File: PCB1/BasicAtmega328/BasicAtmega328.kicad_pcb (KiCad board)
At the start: 2 copper layers, 0 parts

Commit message: Placa enrutada
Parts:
- added C1: 47uF, Capacitors_SMD:CP_Elec_6.3x5.7, F.Cu at (110.5, 97.8)
- added C2: 100nF, Capacitors_SMD:C_0805, F.Cu at (104.1, 78.7)
- added C3: 4.7uF, Capacitors_SMD:C_0805, F.Cu at (102.5, 77.1)
- added C5: 100nF, Capacitors_SMD:C_0805, F.Cu at (113.6, 89.5)
- added C6: 100nF, Capacitors_SMD:C_0805, F.Cu at (97.3, 97.6)
- added C7: 10uF, Capacitors_SMD:C_0805, F.Cu at (118.8, 82.0)
- added C8: 100nF, Capacitors_SMD:C_0805, F.Cu at (118.8, 80.1)
- added D1: MBRA140, Diodes_SMD:D_SMA_Standard, F.Cu at (121.5, 93.0)
- added D2: POWER_ON, LEDs:LED_0805, B.Cu at (113.0, 105.4)
- added D3: SMBJ6.0CA, Diode_SMD:D_SMB, B.Cu at (117.4, 71.3)
- added D4: SMBJ6.0CA, Diode_SMD:D_SMB, B.Cu at (109.1, 71.3)
- added D5: SMBJ6.0CA, Diode_SMD:D_SMB, B.Cu at (100.8, 71.3)
- added F1: 160mA, Fuses:1206, B.Cu at (123.4, 66.4)
- added F2: 160mA, Fuses:1206, B.Cu at (94.7, 66.3)
- added J1: Jack-DC-IN, Connectors:BARREL_JACK, F.Cu at (118.8, 97.0)
- added JP1: VCC_CUT, Jumpers:SMT-JUMPER_2_NO_NO-SILK, B.Cu at (97.5, 84.7)
- added JP2: VCC_CUT, Jumpers:SMT-JUMPER_2_NO_NO-SILK, B.Cu at (119.1, 80.4)
- added JP3: VCC_CUT, Jumpers:SMT-JUMPER_2_NO_NO-SILK, B.Cu at (100.6, 104.3)
- added P1: ISCP, Connectors:2X3, F.Cu at (94.9, 89.3)
- added P2: HEADER1, Pin_Headers:Pin_Header_Straight_1x15, F.Cu at (88.4, 64.2)
- added P3: MODBUS_1, Connectors_Molex:Molex_Microfit3_Header_02x03_Angled_43045-060x, F.Cu at (113.7, 63.4)
- added P4: SERIAL_DEBUG, Connectors_JST:JST_PH_S4B-PH-K_04x2.00mm_Angled, F.Cu at (102.5, 105.0)
- added P5: MODBUS_2, Connectors_Molex:Molex_Microfit3_Header_02x03_Angled_43045-060x, F.Cu at (97.9, 63.4)
- added P6: HEADER2, Pin_Headers:Pin_Header_Straight_1x15, F.Cu at (129.4, 64.4)
- added R1: 1k, Resistors_SMD:R_0805, B.Cu at (113.0, 103.5)
- added R2: 10k, Resistors_SMD:R_0805, F.Cu at (108.1, 74.0)
- added R3: 10k, Resistors_SMD:R_0805, F.Cu at (108.1, 75.9)
- added R4: 1k, Resistors_SMD:R_0805, F.Cu at (98.6, 104.6)
- added R5: 10k, Resistors_SMD:R_0805, F.Cu at (124.1, 73.9)
- added R6: 10k, Resistors_SMD:R_0805, F.Cu at (122.2, 69.8)
- added R7: 10k, Resistors_SMD:R_0805, F.Cu at (111.7, 75.4)
- added R8: 120R(NC), Resistors_SMD:R_0805, B.Cu at (115.3, 73.8)
- added SW1: RESET_Button, Buttons_Switches_SMD:SW_SPST_B3U-3000P, F.Cu at (95.0, 105.1)
- added U1: LM1117-5.0, TO_SOT_Packages_SMD:SOT-223-3_TabPin2, F.Cu at (102.6, 97.9)
- added U2: ATMEGA328P-AU, Housings_QFP:TQFP-32_7x7mm_Pitch0.8mm, F.Cu at (108.1, 84.8)
- added U3: MAX13487E, Housings_SOIC:SO-8_5.3x6.2mm_Pitch1.27mm, F.Cu at (117.9, 75.7)
- added Y1: 16Mhz, Clocks:RESONATOR-SMD-3.2X1.3, F.Cu at (101.2, 81.5)
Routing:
- net +5V: track 0.00 -> 131.6 mm, vias 0 -> 5
- net +12V: track 0.00 -> 102.0 mm, vias 0 -> 3
- net RST: track 0.00 -> 95.8 mm, vias 0 -> 5
- net TXD: track 0.00 -> 59.0 mm, vias 0 -> 2
- net RXD: track 0.00 -> 58.1 mm, vias 0 -> 3
- net 485_TX: track 0.00 -> 49.6 mm, vias 0 -> 3
- net D13-SCK: track 0.00 -> 49.0 mm, vias 0 -> 7
- net 485_RX: track 0.00 -> 41.1 mm, vias 0 -> 2
- net Net-(D4-Pad2): track 0.00 -> 32.3 mm, vias 0 -> 2
- net D12-MISO: track 0.00 -> 31.0 mm
- net D11-MOSI: track 0.00 -> 29.5 mm, vias 0 -> 1
- net Net-(D3-Pad2): track 0.00 -> 28.6 mm, vias 0 -> 3
- net A6: track 0.00 -> 26.0 mm, vias 0 -> 2
- net A7: track 0.00 -> 25.4 mm, vias 0 -> 2
- net D10: track 0.00 -> 25.0 mm
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- added copper zone on B.Cu, net GND
- added copper zone on F.Cu, net GND
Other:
- board outline added: 45 x 49.9 mm

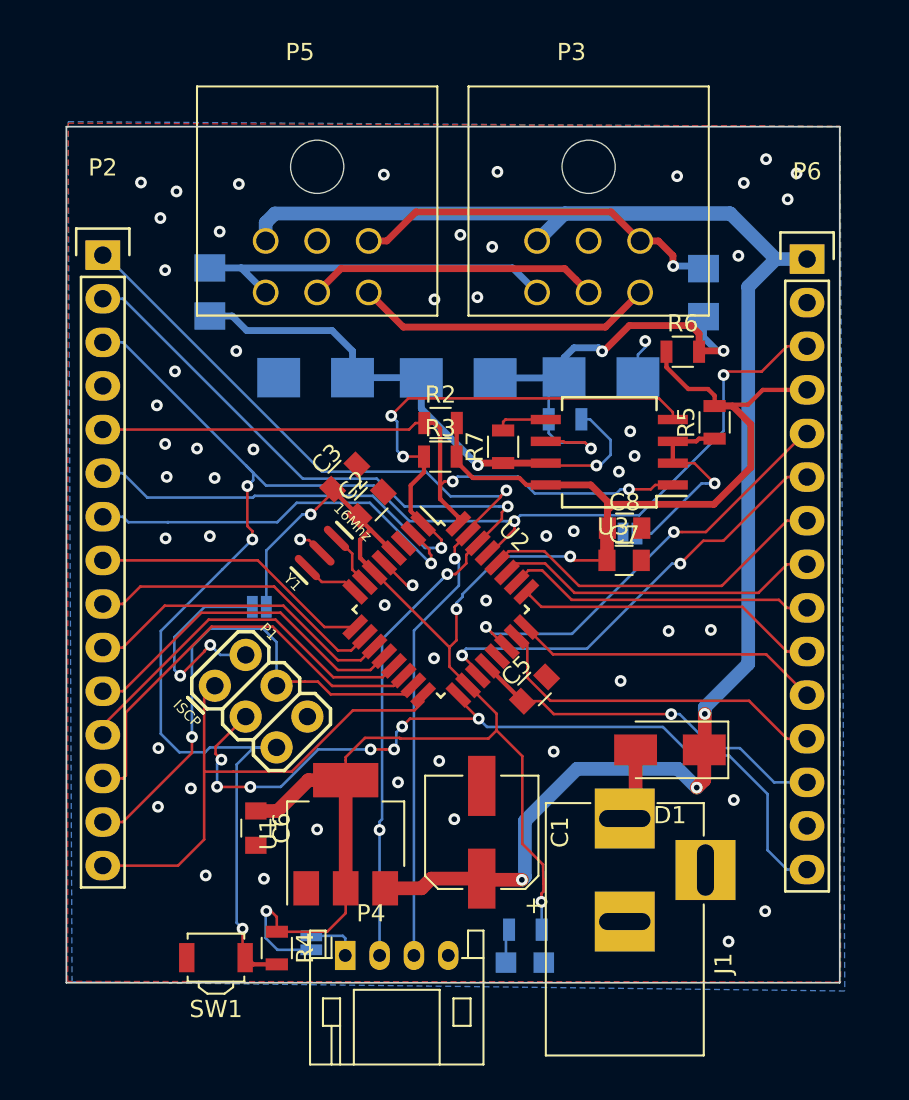
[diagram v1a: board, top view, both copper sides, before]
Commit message: Serigrafia añadida, faltan logos y DRC
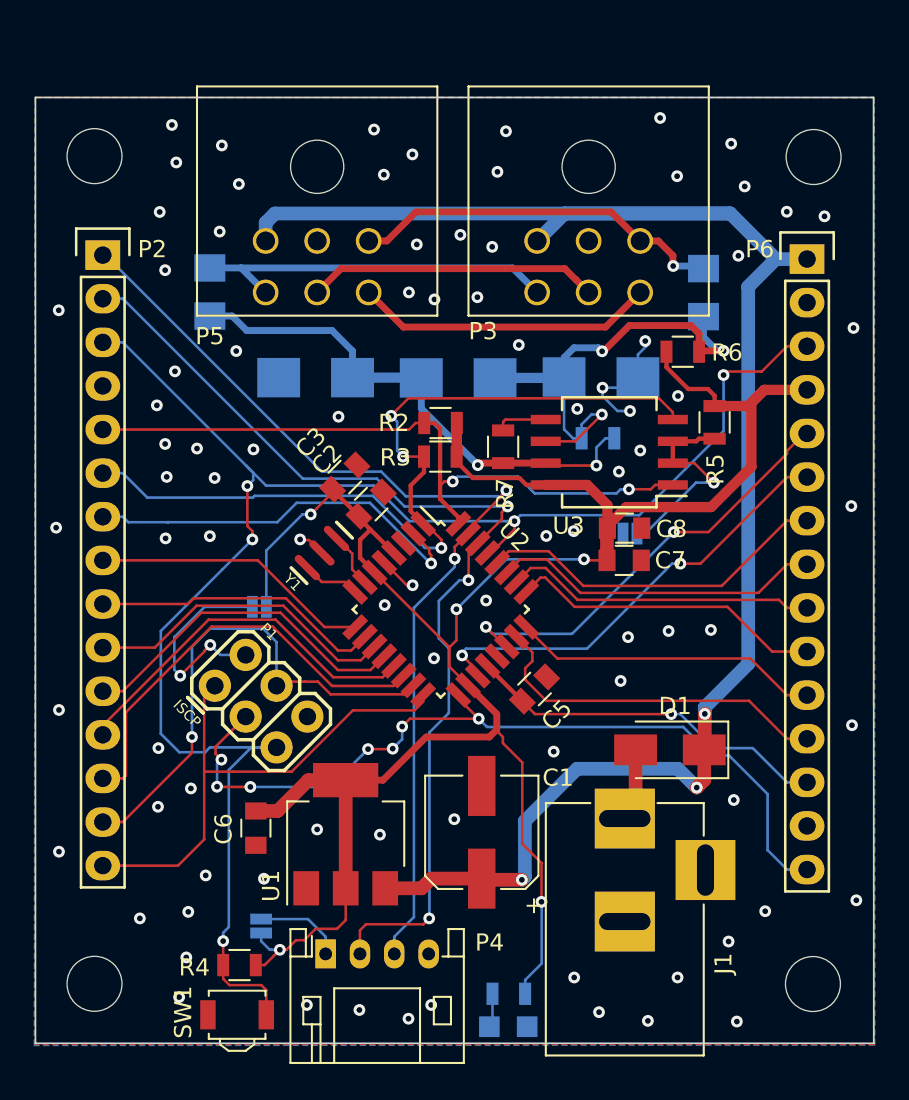
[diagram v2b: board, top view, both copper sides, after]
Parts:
- added REF**: MountingHole_3.2mm_M3, Mounting_Holes:MountingHole_3.2mm_M3, F.Cu at (87.9, 106.6)
- added REF**: MountingHole_3.2mm_M3, Mounting_Holes:MountingHole_3.2mm_M3, F.Cu at (129.8, 106.7)
- added REF**: MountingHole_3.2mm_M3, Mounting_Holes:MountingHole_3.2mm_M3, F.Cu at (129.8, 58.5)
- added REF**: MountingHole_3.2mm_M3, Mounting_Holes:MountingHole_3.2mm_M3, F.Cu at (87.9, 58.4)
- moved D2 3.86 mm to (112.0, 109.1)
- moved R1 3.86 mm to (112.1, 107.2)
- moved SW1 3.55 mm to (96.2, 108.4)
- moved JP3 3.08 mm to (97.6, 103.3)
- moved R4 2.39 mm to (96.4, 105.5), turned to 180 degrees
- moved R8 2.21 mm to (117.3, 74.9)
- moved P4 1.15 mm to (101.4, 104.9)
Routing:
- net +5V: track 131.6 -> 142.3 mm
- net GND: track 9.15 -> 13.9 mm, vias 55 -> 88
- net RST: track 95.8 -> 99.5 mm
- net RXD: track 58.1 -> 61.1 mm
- net Net-(D3-Pad2): track 28.6 -> 31.1 mm
- net Net-(JP3-Pad2): track 3.04 -> 5.19 mm
- net Net-(D4-Pad2): track 32.3 -> 30.6 mm
- net A2: track 17.8 -> 18.5 mm
- net D6: track 17.6 -> 17.0 mm
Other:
- board size 45 x 49.9 mm -> 48.8 x 55.1 mm
- board text added: "BasicAtmega V0.1"
